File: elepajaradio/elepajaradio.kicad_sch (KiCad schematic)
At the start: 34 parts, among them Q1 2N2219, Q2 2N2219, SW1 RotaryEncoder, U1 ATmega328P-A, U2 OLED_I2C, U3 Opamp_Dual, Y1 Crystal

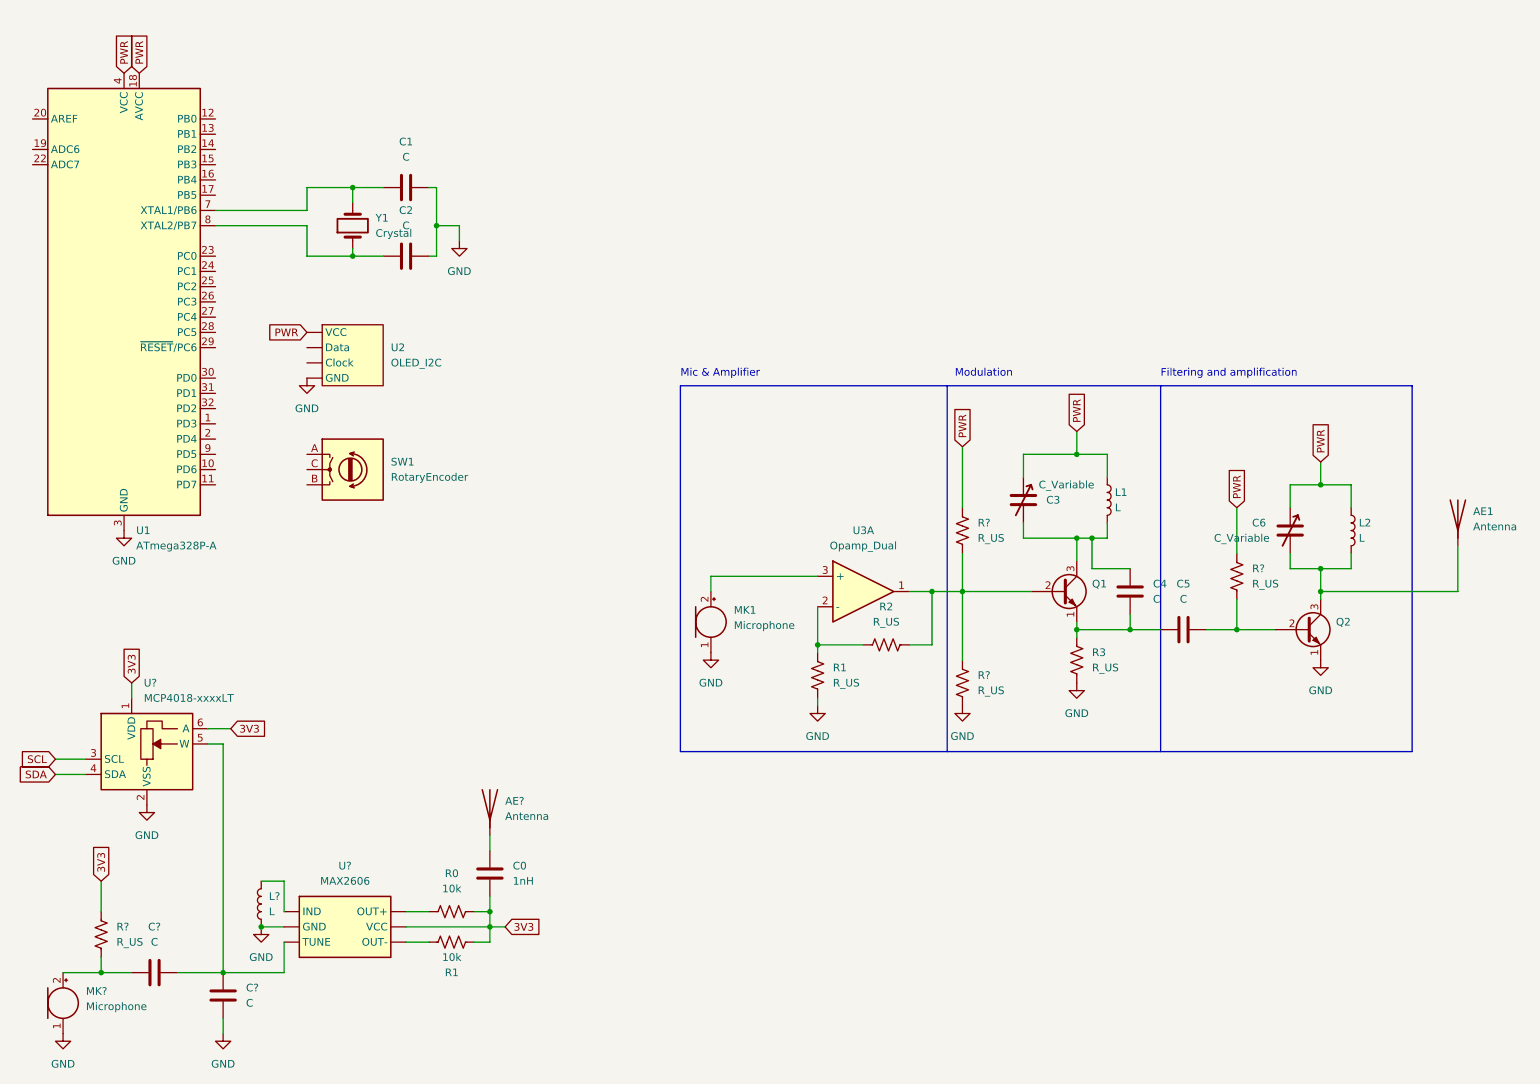
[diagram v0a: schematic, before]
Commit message: MCU
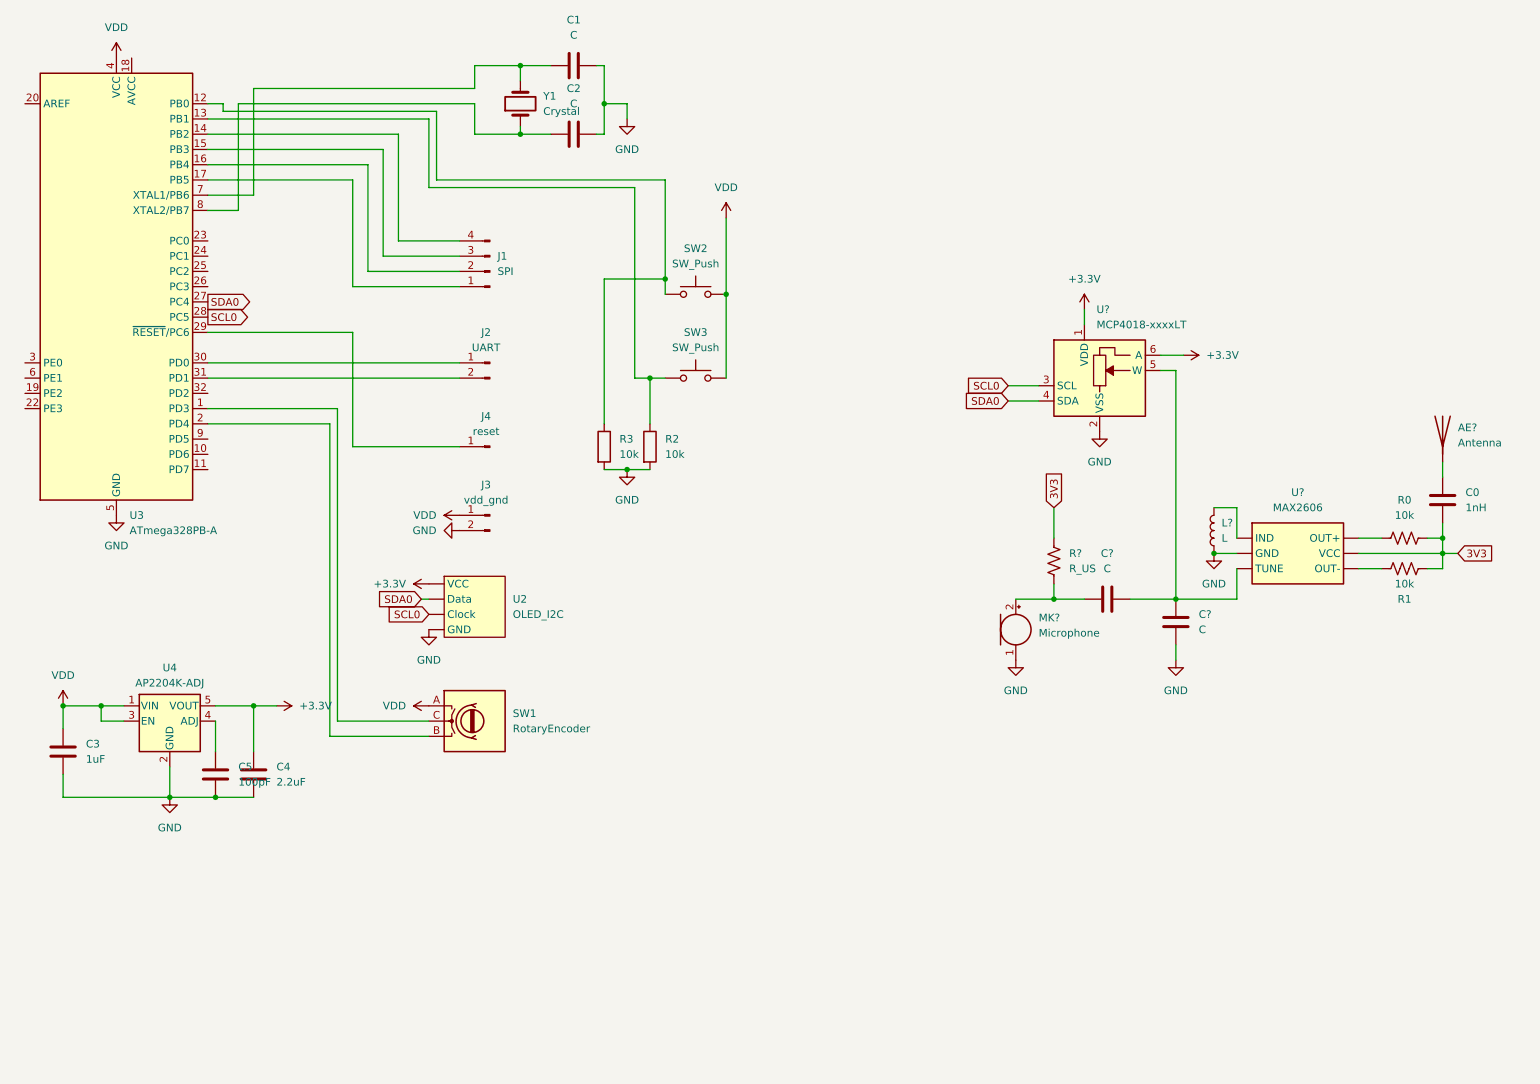
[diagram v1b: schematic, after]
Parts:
- removed AE1: Antenna, symbol Device:Antenna
- removed C3, C6: C_Variable, symbol Device:C_Variable
- removed L1, L2: L, symbol Device:L
- removed MK1: Microphone, symbol Device:Microphone
- removed Q1, Q2: 2N2219, Package_TO_SOT_THT:TO-39-3, symbol Transistor_BJT:2N2219
- removed R1, R2, R3, R? (x3): R_US, symbol Device:R_US
- removed U1: ATmega328P-A, Package_QFP:TQFP-32_7x7mm_P0.8mm, symbol MCU_Microchip_ATmega:ATmega328P-A
- removed U3: Opamp_Dual, symbol Device:Opamp_Dual
- added C3: 1uF, symbol Device:C
- added J1: SPI, symbol Connector:Conn_01x04_Pin
- added J2: UART, symbol Connector:Conn_01x02_Pin
- added J3: vdd_gnd, symbol Connector:Conn_01x02_Pin
- added J4: reset, symbol Connector:Conn_01x01_Pin
- added R2, R3: 10k, symbol Device:R
- added SW2, SW3: SW_Push, symbol Switch:SW_Push
- added U3: ATmega328PB-A, Package_QFP:TQFP-32_7x7mm_P0.8mm, symbol MCU_Microchip_ATmega:ATmega328PB-A
- added U4: AP2204K-ADJ, Package_TO_SOT_SMD:SOT-23-5, symbol Regulator_Linear:AP2204K-ADJ
- C4: value C -> 2.2uF
- C5: value C -> 100pF
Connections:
- net PWR is gone; now on net SDA0: U2. (VCC)
- net SDA is gone; now on net SDA0: U?.4 (SDA)
- net 3V3: no longer U?.1 (VDD), U?.6 (A)
- net GND: now also C4.2, C5.2, C3.2, J3.2 (Pin_2), R2.2, R3.2, U3.21 (GND), U3.5 (GND), U4.2 (GND)
- net SDA0: now reaches U2. (VCC)
- net SDA0: now also U3.27 (PC4)
- net +3.3V: now reaches C4.1
- net +3.3V: now also U2. (VCC), U?.1 (VDD), U?.6 (A), U4.5 (VOUT)
- net at C2.1, Y1.1: now also U3.8 (XTAL2/PB7)
- net at C1.1, Y1.2: now also U3.7 (XTAL1/PB6)
- net at C5.1: now also U4.4 (ADJ); no longer C4.2
- net VDD: now reaches SW1.A
- net VDD: now also C3.1, J3.1 (Pin_1), SW2.2, SW3.2, U3.4 (VCC), U4.1 (VIN), U4.3 (EN)
- net at SW1.B: now also U3.2 (PD4)
- net at SW1.C: now also U3.1 (PD3)
- net SCL renamed SCL0
- net SCL0: now also U2. (VCC), U3.28 (PC5)
- new net: J1.1 (Pin_1), U3.17 (PB5)
- new net: J1.2 (Pin_2), U3.16 (PB4)
- new net: J1.3 (Pin_3), U3.15 (PB3)
- new net: J1.4 (Pin_4), U3.14 (PB2)
- new net: J2.1 (Pin_1), U3.30 (PD0)
- new net: J2.2 (Pin_2), U3.31 (PD1)
- new net: J4.1 (Pin_1), U3.29 (~{RESET}/PC6)
- new net: R2.1, SW3.1, U3.13 (PB1)
- new net: R3.1, SW2.1, U3.12 (PB0)
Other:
- note removed: "Filtering and amplification"
- note removed: "Mic & Amplifier"
- note removed: "Modulation"
- moved on the sheet: AE?, C0, C1, C2, C?, L?, MK?, R0, R1, R?, SW1, U2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
